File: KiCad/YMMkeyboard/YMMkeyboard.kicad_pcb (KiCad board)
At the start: 2 copper layers, 62 parts, among them SW10 SW_Push, SW11 SW_Push, SW12 SW_Push, SW13 SW_Push, SW14 SW_Push, SW15 SW_Push, SW16 SW_Push, SW17 SW_Push, SW18 SW_Push, SW19 SW_Push, SW2 SW_Push, SW20 SW_Push, SW21 SW_Push, SW22 SW_Push, SW23 SW_Push, SW24 SW_Push, SW25 SW_Push, SW26 SW_Push, SW27 SW_Push, SW28 SW_Push, SW29 SW_Push, SW3 SW_Push, SW30 SW_Push, SW31 SW_Push, SW32 RotaryEncoder_Switch, SW4 SW_Push, SW5 SW_Push, SW6 SW_Push, SW7 SW_Push, SW8 SW_Push, SW9 SW_Push

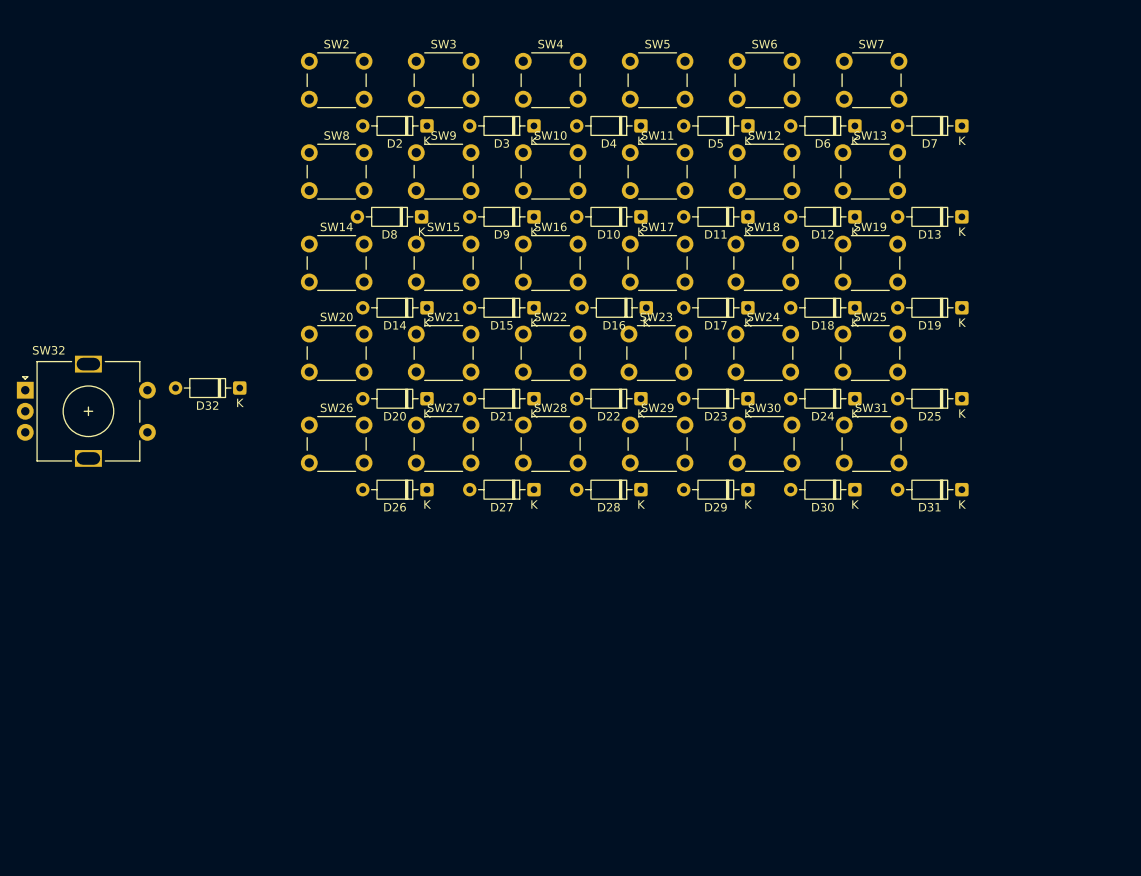
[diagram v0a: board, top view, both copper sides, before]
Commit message: 2号機発注データ
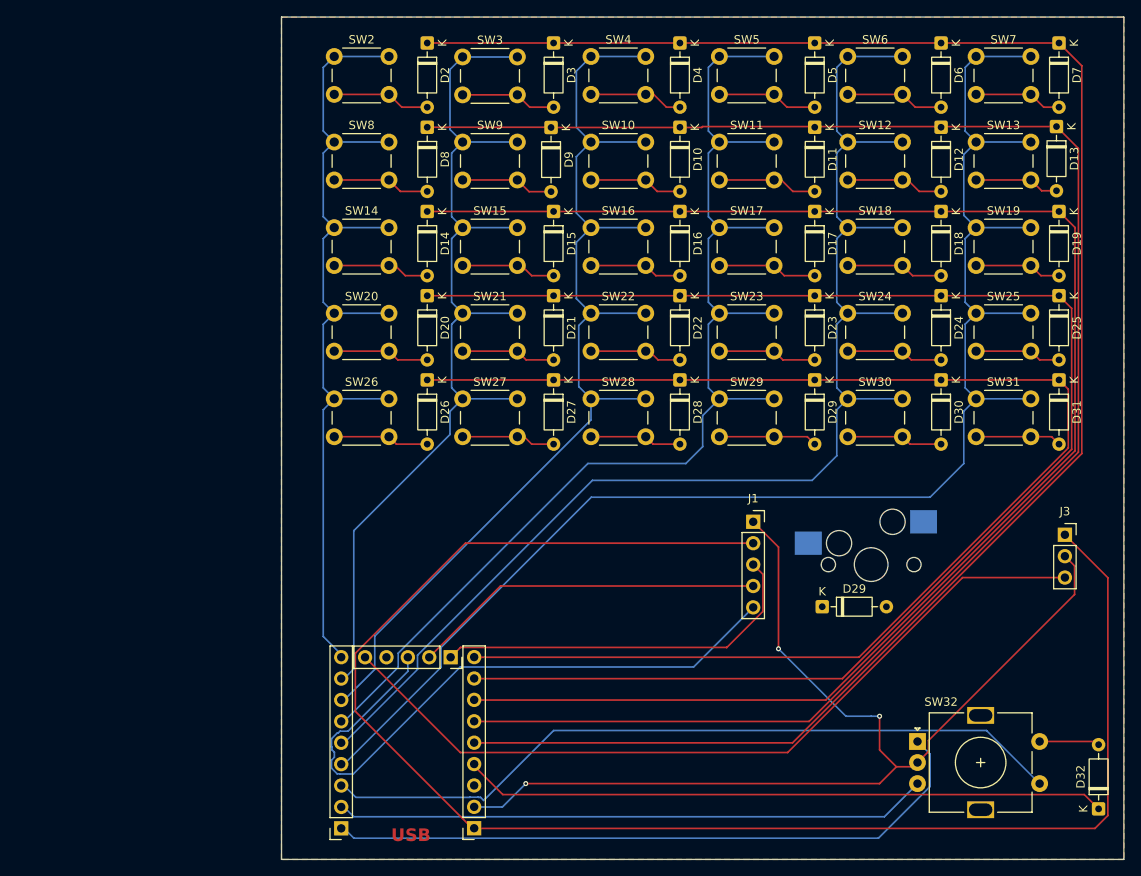
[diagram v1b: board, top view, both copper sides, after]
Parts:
- removed the D29 at (166.4, 78.1)
- added D29: 1N4148, Diode_THT:D_DO-35_SOD27_P7.62mm_Horizontal, F.Cu at (175.2, 92.0)
- added D29: 1N4148, Diode_THT:D_DO-35_SOD27_P7.62mm_Horizontal, F.Cu at (174.3, 65.1)
- added J1: OLED, Connector_PinSocket_2.54mm:PinSocket_1x05_P2.54mm_Vertical, F.Cu at (167.0, 81.9)
- added J3: RGB, Connector_PinSocket_2.54mm:PinSocket_1x03_P2.54mm_Vertical, F.Cu at (204.0, 83.5)
- added REF**: KEY_SWITCH, isw-kbd:CherryMX_Hotswap_1u, F.Cu at (181.0, 87.0)
- added U1: RP2040-Zero, RP2040-ZeroSocket:RP2040-ZeroSocket, F.Cu at (125.7, 108.3)
- moved SW32 113.8 mm to (186.5, 108.0)
- moved D32 113.5 mm to (208.0, 116.0), turned to 90 degrees
- moved D31 17.4 mm to (203.3, 65.1), turned to -90 degrees
- moved D25 16.8 mm to (203.3, 55.1), turned to -90 degrees
- moved D30 16.6 mm to (189.3, 65.1), turned to -90 degrees
- moved D19 16.2 mm to (203.3, 45.1), turned to -90 degrees
- moved SW25 16.0 mm to (193.5, 57.2)
- moved SW31 16.0 mm to (193.5, 67.3)
- moved D24 15.9 mm to (189.3, 55.1), turned to -90 degrees
- moved SW19 15.9 mm to (193.5, 47.0)
- moved SW13 15.9 mm to (193.5, 36.8)
- moved SW7 15.7 mm to (193.5, 26.7)
- moved D13 15.5 mm to (203.0, 35.0), turned to -90 degrees
- moved D18 15.3 mm to (189.3, 45.1), turned to -90 degrees
- moved D7 15.2 mm to (203.3, 25.1), turned to -90 degrees
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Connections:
- D11 pad 1: Net-(D11-K) -> Net-(D10-K)
- D11 pad 2: Net-(D10-K) -> Net-(D11-A)
- D12 pad 1: Net-(D12-K) -> Net-(D10-K)
- D12 pad 2: Net-(D11-K) -> Net-(D12-A)
- D13 pad 1: Net-(D13-K) -> Net-(D10-K)
- D13 pad 2: Net-(D12-K) -> Net-(D13-A)
- D15 pad 1: Net-(D15-K) -> Net-(D14-K)
- D15 pad 2: Net-(D14-K) -> Net-(D15-A)
- D16 pad 1: Net-(D16-K) -> Net-(D14-K)
- D16 pad 2: Net-(D15-K) -> Net-(D16-A)
- D17 pad 1: Net-(D17-K) -> Net-(D14-K)
- D17 pad 2: Net-(D16-K) -> Net-(D17-A)
- D18 pad 1: Net-(D18-K) -> Net-(D14-K)
- D18 pad 2: Net-(D17-K) -> Net-(D18-A)
- D19 pad 1: Net-(D19-K) -> Net-(D14-K)
- D19 pad 2: Net-(D18-K) -> Net-(D19-A)
- D21 pad 1: Net-(D21-K) -> Net-(D20-K)
- D21 pad 2: Net-(D20-K) -> Net-(D21-A)
- D22 pad 1: Net-(D22-K) -> Net-(D20-K)
- D22 pad 2: Net-(D21-K) -> Net-(D22-A)
- D23 pad 1: Net-(D23-K) -> Net-(D20-K)
- D23 pad 2: Net-(D22-K) -> Net-(D23-A)
- D24 pad 1: Net-(D24-K) -> Net-(D20-K)
- D24 pad 2: Net-(D23-K) -> Net-(D24-A)
- D25 pad 1: Net-(D25-K) -> Net-(D20-K)
- D25 pad 2: Net-(D24-K) -> Net-(D25-A)
- D27 pad 1: Net-(D27-K) -> Net-(D26-K)
- D27 pad 2: Net-(D26-K) -> Net-(D27-A)
- D28 pad 1: Net-(D28-K) -> Net-(D26-K)
- D28 pad 2: Net-(D27-K) -> Net-(D28-A)
- D3 pad 1: Net-(D3-K) -> Net-(D2-K)
- D3 pad 2: Net-(D2-K) -> Net-(D3-A)
- D30 pad 1: Net-(D30-K) -> Net-(D26-K)
- D31 pad 1: Net-(D31-K) -> Net-(D26-K)
- D31 pad 2: Net-(D30-K) -> Net-(D31-A)
- D4 pad 1: Net-(D4-K) -> Net-(D2-K)
- D4 pad 2: Net-(D3-K) -> Net-(D4-A)
- D5 pad 1: Net-(D5-K) -> Net-(D2-K)
- D5 pad 2: Net-(D4-K) -> Net-(D5-A)
- D6 pad 1: Net-(D6-K) -> Net-(D2-K)
- D6 pad 2: Net-(D5-K) -> Net-(D6-A)
- D7 pad 1: Net-(D7-K) -> Net-(D2-K)
- D7 pad 2: Net-(D6-K) -> Net-(D7-A)
- D8 pad 1: Net-(D8-K) -> Net-(D10-K)
- D9 pad 1: Net-(D10-A) -> Net-(D10-K)
- D9 pad 2: Net-(D8-K) -> Net-(D9-A)
- SW11 pad 2: Net-(D10-K) -> Net-(D11-A)
- SW12 pad 2: Net-(D11-K) -> Net-(D12-A)
- SW13 pad 2: Net-(D12-K) -> Net-(D13-A)
- SW15 pad 2: Net-(D14-K) -> Net-(D15-A)
- SW16 pad 2: Net-(D15-K) -> Net-(D16-A)
- SW17 pad 2: Net-(D16-K) -> Net-(D17-A)
- SW18 pad 2: Net-(D17-K) -> Net-(D18-A)
- SW19 pad 2: Net-(D18-K) -> Net-(D19-A)
- SW21 pad 2: Net-(D20-K) -> Net-(D21-A)
- SW22 pad 2: Net-(D21-K) -> Net-(D22-A)
- SW23 pad 2: Net-(D22-K) -> Net-(D23-A)
- SW24 pad 2: Net-(D23-K) -> Net-(D24-A)
- SW25 pad 2: Net-(D24-K) -> Net-(D25-A)
- SW27 pad 2: Net-(D26-K) -> Net-(D27-A)
- SW28 pad 2: Net-(D27-K) -> Net-(D28-A)
- SW29 pad 2: Net-(D28-K) -> Net-(D29-A)
- SW3 pad 2: Net-(D2-K) -> Net-(D3-A)
- SW31 pad 2: Net-(D30-K) -> Net-(D31-A)
- SW4 pad 2: Net-(D3-K) -> Net-(D4-A)
- SW5 pad 2: Net-(D4-K) -> Net-(D5-A)
- SW6 pad 2: Net-(D5-K) -> Net-(D6-A)
- SW7 pad 2: Net-(D6-K) -> Net-(D7-A)
- SW9 pad 2: Net-(D8-K) -> Net-(D9-A)
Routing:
- net Net-(D2-K): track 0.00 -> 211.4 mm
- net Net-(D10-K): track 0.00 -> 199.7 mm
- net Net-(J1-Pin_2): track 0.00 -> 190.7 mm
- net Net-(D14-K): track 0.00 -> 188.0 mm
- net Net-(D20-K): track 0.00 -> 176.3 mm
- net Net-(SW13-Pad1): track 0.00 -> 175.6 mm
- net Net-(D26-K): track 0.00 -> 164.6 mm
- net Net-(SW12-Pad1): track 0.00 -> 158.3 mm
- net Net-(SW11-Pad1): track 0.00 -> 141.0 mm
- net Net-(SW10-Pad1): track 0.00 -> 126.6 mm
- net GND: track 0.00 -> 126.2 mm, vias 0 -> 3
- net Net-(SW15-Pad1): track 0.00 -> 116.6 mm
- net Net-(SW14-Pad1): track 0.00 -> 109.7 mm
- net Net-(J3-Pin_3): track 0.00 -> 96.4 mm
- net Net-(SW32-PadS1): track 0.00 -> 89.4 mm
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- added copper zone on F.Cu, net (none)
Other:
- board outline added: 100 x 100 mm
- board text added: "USB"
